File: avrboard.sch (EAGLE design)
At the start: 11 parts, among them IC1 MEGA48/88/168-AU, IC2 78L05SMD

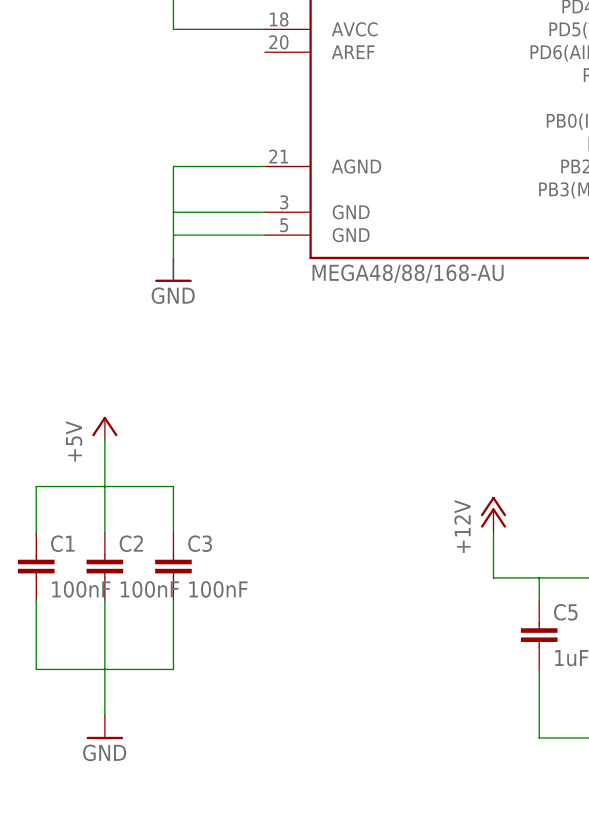
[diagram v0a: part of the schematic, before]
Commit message: updated readme, small fixes on schema
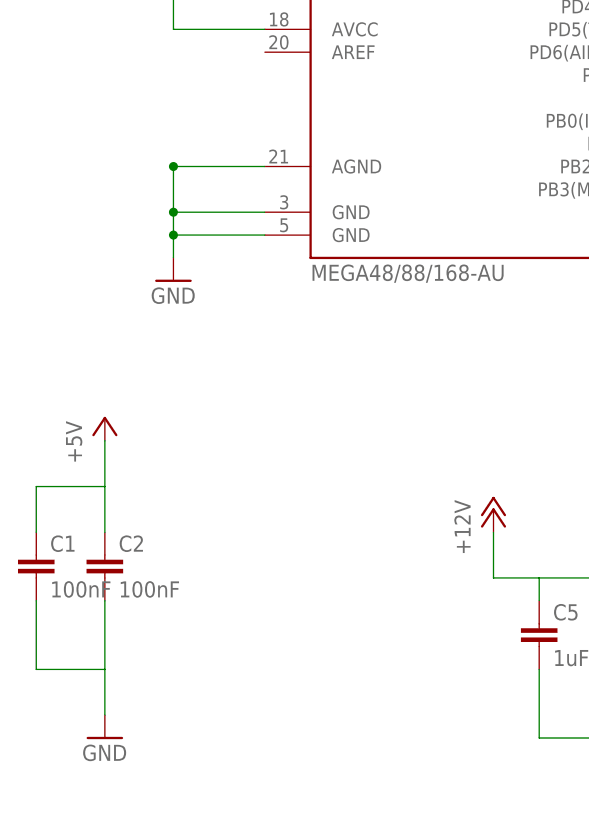
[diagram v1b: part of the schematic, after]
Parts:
- removed C3: 100nF, rcl:C-EUC0805
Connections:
- removed net N$1: IC1.AGND, IC1.GND@1, IC1.GND@2
- net +5V: no longer C3.1
- net GND: now also IC1.AGND, IC1.GND@1, IC1.GND@2; no longer C3.2
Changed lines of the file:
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@@
 <part name="C1" library="rcl" deviceset="C-EU" device="C0805" value="100nF"/>
 <part name="C2" library="rcl" deviceset="C-EU" device="C0805" value="100nF"/>
-<part name="C3" library="rcl" deviceset="C-EU" device="C0805" value="100nF"/>
 <part name="IC2" library="linear" deviceset="78L*SMD" device="" technology="05"/>
 <part name="C4" library="rcl" deviceset="C-EU" device="C0805" value="100nF"/>
@@
 <instance part="C1" gate="G$1" x="12.7" y="38.1"/>
 <instance part="C2" gate="G$1" x="20.32" y="38.1"/>
-<instance part="C3" gate="G$1" x="27.94" y="38.1"/>
 <instance part="IC2" gate="G$1" x="88.9" y="35.56"/>
 <instance part="C4" gate="G$1" x="111.76" y="33.02"/>
@@
 </segment>
 <segment>
-<pinref part="C3" gate="G$1" pin="1"/>
-<wire x1="27.94" y1="40.64" x2="27.94" y2="45.72" width="0.1524" layer="91"/>
-<wire x1="27.94" y1="45.72" x2="20.32" y2="45.72" width="0.1524" layer="91"/>
 <pinref part="C1" gate="G$1" pin="1"/>
 <wire x1="20.32" y1="45.72" x2="12.7" y2="45.72" width="0.1524" layer="91"/>
@@
 <wire x1="12.7" y1="33.02" x2="12.7" y2="25.4" width="0.1524" layer="91"/>
 <wire x1="12.7" y1="25.4" x2="20.32" y2="25.4" width="0.1524" layer="91"/>
-<pinref part="C3" gate="G$1" pin="2"/>
-<wire x1="20.32" y1="25.4" x2="27.94" y2="25.4" width="0.1524" layer="91"/>
-<wire x1="27.94" y1="25.4" x2="27.94" y2="33.02" width="0.1524" layer="91"/>
 <pinref part="C2" gate="G$1" pin="2"/>
 <wire x1="20.32" y1="33.02" x2="20.32" y2="25.4" width="0.1524" layer="91"/>
@@
 <wire x1="20.32" y1="20.32" x2="20.32" y2="25.4" width="0.1524" layer="91"/>
 </segment>
-</net>
-<net name="N$1" class="0">
 <segment>
 <pinref part="IC1" gate="1" pin="GND@2"/>
 <wire x1="38.1" y1="73.66" x2="27.94" y2="73.66" width="0.1524" layer="91"/>
-<wire x1="27.94" y1="73.66" x2="27.94" y2="68.58" width="0.1524" layer="91"/>
+<wire x1="27.94" y1="73.66" x2="27.94" y2="71.12" width="0.1524" layer="91"/>
 <pinref part="IC1" gate="1" pin="GND@1"/>
 <wire x1="38.1" y1="76.2" x2="27.94" y2="76.2" width="0.1524" layer="91"/>
@@
 <wire x1="38.1" y1="81.28" x2="27.94" y2="81.28" width="0.1524" layer="91"/>
 <wire x1="27.94" y1="81.28" x2="27.94" y2="76.2" width="0.1524" layer="91"/>
+<junction x="27.94" y="81.28"/>
+<junction x="27.94" y="76.2"/>
+<junction x="27.94" y="73.66"/>
 </segment>
 </net>
